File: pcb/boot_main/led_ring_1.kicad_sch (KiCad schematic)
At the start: 10 parts, among them Q1 NPN

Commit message: Assign footprints
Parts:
- D1, D2, D3, D4: footprint (none) -> LED_SMD:LED_1206_3216Metric
- Q1: footprint (none) -> Package_TO_SOT_SMD:SOT-323_SC-70
- R15, R16, R17, R18, R19: footprint (none) -> Resistor_SMD:R_0603_1608Metric
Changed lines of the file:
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@@
 			)
 		)
-		(property "Footprint" ""
+		(property "Footprint" "Resistor_SMD:R_0603_1608Metric"
 			(at 170.942 86.36 90)
 			(effects
@@
 			)
 		)
-		(property "Footprint" ""
+		(property "Footprint" "Resistor_SMD:R_0603_1608Metric"
 			(at 160.782 86.36 90)
 			(effects
@@
 			)
 		)
-		(property "Footprint" ""
+		(property "Footprint" "LED_SMD:LED_1206_3216Metric"
 			(at 152.4 96.52 0)
 			(effects
@@
 			)
 		)
-		(property "Footprint" ""
+		(property "Footprint" "LED_SMD:LED_1206_3216Metric"
 			(at 162.56 96.52 0)
 			(effects
@@
 			)
 		)
-		(property "Footprint" ""
+		(property "Footprint" "Package_TO_SOT_SMD:SOT-323_SC-70"
 			(at 203.2 110.49 0)
 			(effects
@@
 			)
 		)
-		(property "Footprint" ""
+		(property "Footprint" "Resistor_SMD:R_0603_1608Metric"
 			(at 150.622 86.36 90)
 			(effects
@@
 			)
 		)
-		(property "Footprint" ""
+		(property "Footprint" "LED_SMD:LED_1206_3216Metric"
 			(at 172.72 96.52 0)
 			(effects
@@
 			)
 		)
-		(property "Footprint" ""
+		(property "Footprint" "Resistor_SMD:R_0603_1608Metric"
 			(at 128.27 112.268 90)
 			(effects
@@
 			)
 		)
-		(property "Footprint" ""
+		(property "Footprint" "LED_SMD:LED_1206_3216Metric"
 			(at 142.24 96.52 0)
 			(effects
@@
 			)
 		)
-		(property "Footprint" ""
+		(property "Footprint" "Resistor_SMD:R_0603_1608Metric"
 			(at 140.462 86.36 90)
 			(effects

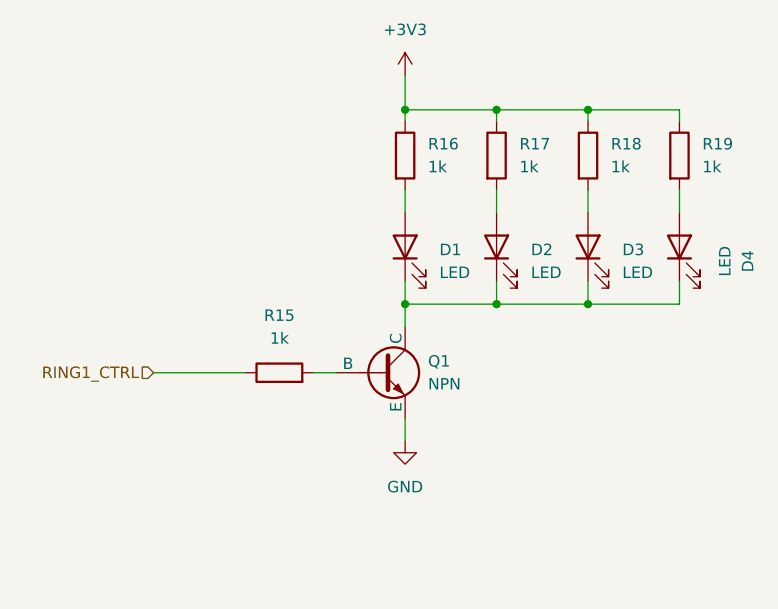
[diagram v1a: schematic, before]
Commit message: MOre layout
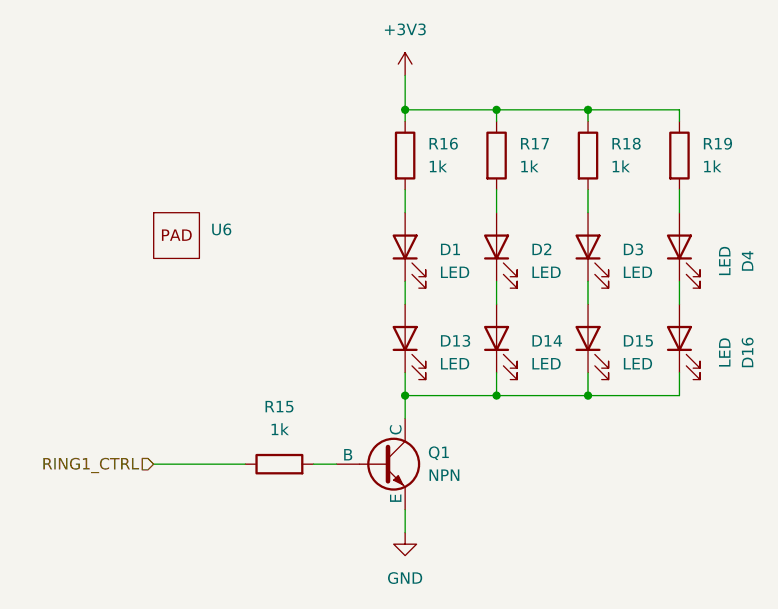
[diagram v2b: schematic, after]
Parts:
- added D13, D14, D15, D16: LED, LED_SMD:LED_1206_3216Metric, symbol Device:LED
- added U6: ~, cap_pads:square_20x20mm_guide, symbol cap_pads:capacitive_pad_guide
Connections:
- new net: D13.1 (K), D14.1 (K), D15.1 (K), D16.1 (K), Q1.1 (C)
- new net: D14.2 (A), D2.1 (K)
- new net: D15.2 (A), D3.1 (K)
- new net: D16.2 (A), D4.1 (K)
- new net: D1.1 (K), D13.2 (A)
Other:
- moved on the sheet: Q1, R15
